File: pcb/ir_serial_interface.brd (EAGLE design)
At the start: 41.6 x 43.2 mm, 24 parts, among them IC1 PIC18F2550_28W, Q1 BSS123, T1 SFH303

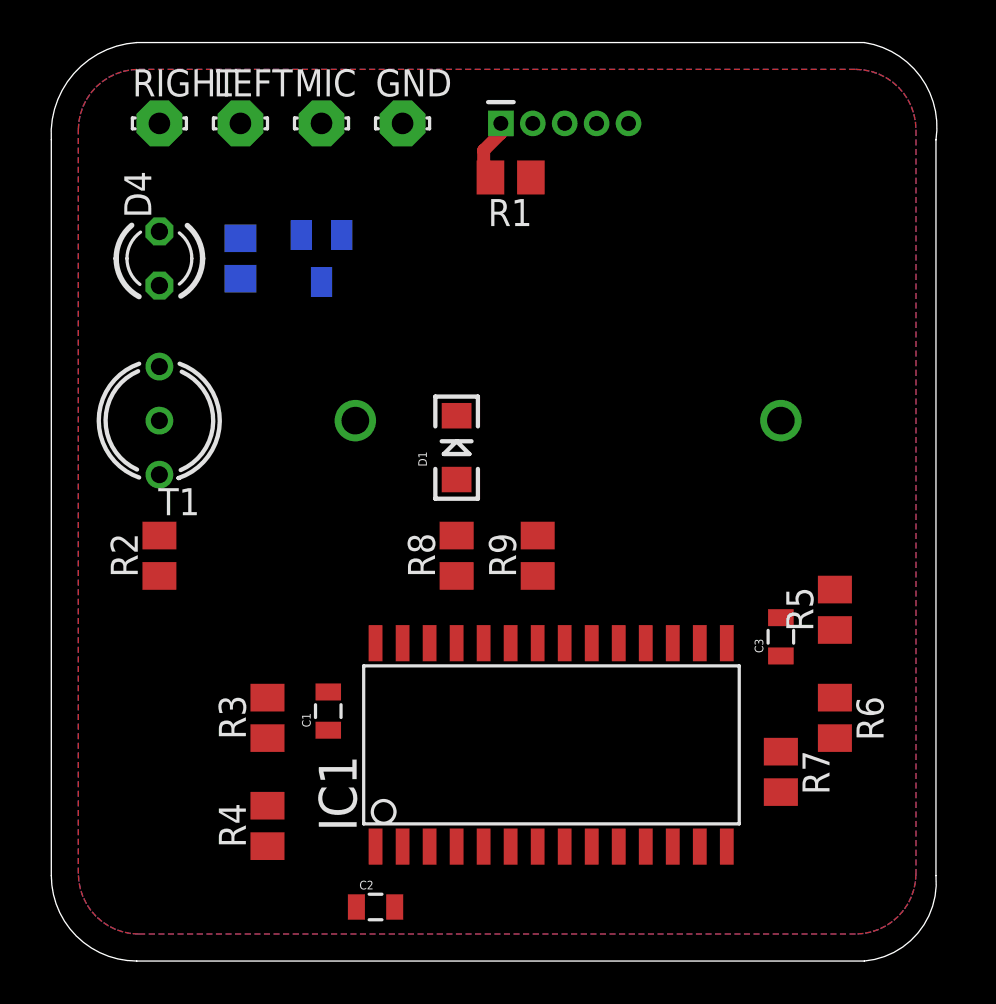
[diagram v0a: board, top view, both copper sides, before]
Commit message: PCB: board layout done
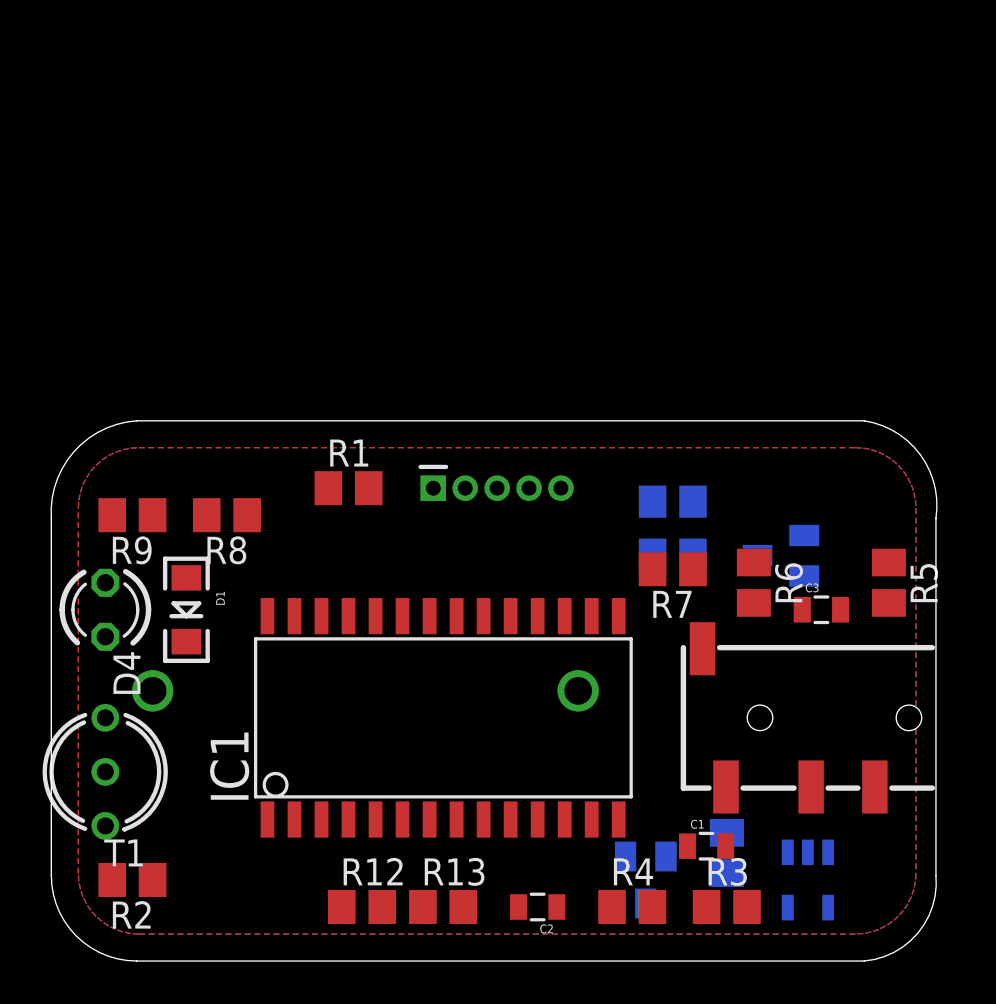
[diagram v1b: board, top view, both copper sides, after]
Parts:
- removed GND, LEFT, MIC, RIGHT: LSP10, solpad:LSP10
- removed Q1: BSS123, transistor-small-signal:SOT23
- added D2: (no value), semicon-smd-ipc:SOT23
- added IC2: LP2992, texas:SOT23-DBV
- added Q2: BC847SMD, transistor-npn:SOT23
- added R10: 2k, resistor:M0805
- added R11, R12, R13: 100k, resistor:M0805
- added U$2: AUDIO-JACK3, SparkFun-Connectors:AUDIO-JACK-TRRS-SMD
- moved R3 23.3 mm to (53.3, 27.9), turned to 0 degrees
- moved C4 23.3 mm to (50.8, 47.0), turned to 0 degrees
- moved R9 19.1 mm to (25.4, 46.4), turned to 180 degrees
- moved C1 18.9 mm to (52.4, 30.8), turned to 0 degrees
- moved R4 17.6 mm to (48.9, 27.9), turned to 0 degrees
- moved U$1 17.4 mm to (42.5, 47.6)
- moved D4 16.7 mm to (24.1, 41.9), turned to 270 degrees
- moved T1 16.7 mm to (24.1, 34.3)
- moved R1 16.5 mm to (35.6, 47.6), turned to 0 degrees
- moved BAT1 15.9 mm to (46.4, 38.1)
- moved R2 15.3 mm to (25.4, 29.2), turned to 180 degrees
- moved D1 14.8 mm to (27.9, 41.9), turned to 270 degrees
- moved R8 11.0 mm to (29.8, 46.4), turned to 180 degrees
- moved R7 10.8 mm to (50.8, 43.8), turned to 180 degrees
- moved C2 7.62 mm to (44.5, 27.9), turned to 180 degrees
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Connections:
- removed net -: BAT1.2
- new net N$12: D2.1, U$2.RING1
- new net N$13: IC2.3, Q2.2, R11.1
- new net N$18: C4.1, D2.3, R10.2
- new net V+: BAT1.1, IC2.1, Q2.3, R13.2
- net +5V: now also IC2.5; no longer Q1.2
- net GND: now also BAT1.2, IC2.2, R11.2, R12.1, U$2.RING2; no longer GND.MP
- net N$16: now also IC1.7, R12.2, R13.1; no longer BAT1.1, Q1.3
- net N$17: now also Q2.1, R10.1; no longer C4.1, Q1.1, RIGHT.MP
- net N$5: now also U$2.TIP; no longer LEFT.MP
- net N$7: now also U$2.EARTH; no longer MIC.MP
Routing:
- net N$2: track 3.01 -> 0.00 mm
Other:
- board size 41.6 x 43.2 mm -> 41.6 x 25.4 mm
